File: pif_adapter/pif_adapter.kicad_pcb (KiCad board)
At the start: 2 copper layers, 11 x 22 mm, 11 parts, among them P1 Conn_02x20_Odd_Even, P10 Conn_01x01, P11 Conn_01x01, P2 PIF-NUS, P3 Conn_01x01, P4 Conn_01x01, P5 Conn_01x01, P6 Conn_01x01, P7 Conn_01x01, P8 Conn_01x01, P9 Conn_01x01

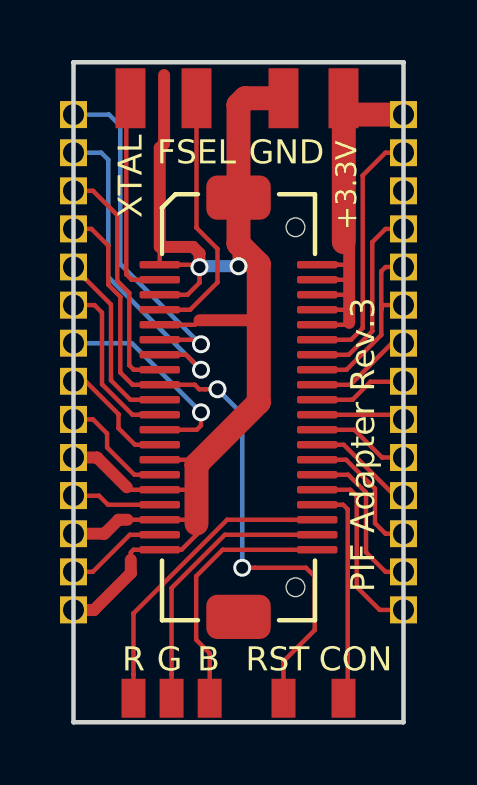
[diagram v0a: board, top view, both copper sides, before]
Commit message: - updated revision infos - changed some traces
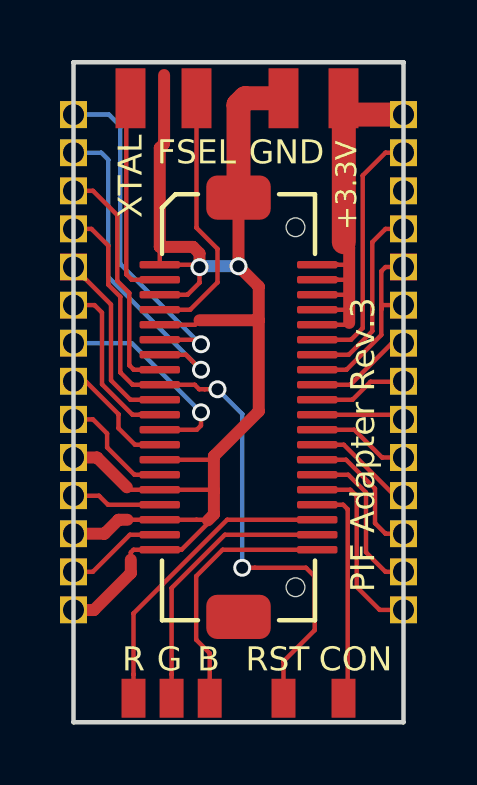
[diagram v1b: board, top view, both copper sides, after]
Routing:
- net GND: track 51.8 -> 51.1 mm
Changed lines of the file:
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@@
     (thickness 1.6)
     (drawings 20)
-    (tracks 221)
+    (tracks 222)
     (zones 0)
     (modules 11)
@@
   )
   (page A4)
+  (title_block
+    (title "UltraPIF Adapter")
+    (date 2020-03-04)
+    (rev 3)
+  )
   (layers
     (0 F.Cu signal)
@@
   )
   (setup
-    (last_trace_width 0.8)
+    (last_trace_width 0.4)
     (user_trace_width 0.4)
     (user_trace_width 0.8)
@@
   (segment (start 143.03 109.25) (end 142.12 108.34) (width 0.15) (layer F.Cu) (net 9))
   (segment (start 141.01 111.225) (end 141 111.215) (width 0.15) (layer F.Cu) (net 10))
-  (segment (start 143.975 110.75) (end 142.8 110.75) (width 0.15) (layer F.Cu) (net 10))
   (segment (start 141 111.215) (end 142.035 111.215) (width 0.4) (layer F.Cu) (net 10))
   (segment (start 142.5 110.75) (end 142.8 110.75) (width 0.4) (layer F.Cu) (net 10))
   (segment (start 142.035 111.215) (end 142.5 110.75) (width 0.4) (layer F.Cu) (net 10))
-  (segment (start 143.975 108.75) (end 144.925 108.75) (width 0.15) (layer F.Cu) (net 10))
   (via (at 146.5 102.3) (size 0.6) (drill 0.4) (layers F.Cu B.Cu) (net 10))
   (segment (start 145.2 102.3) (end 146.5 102.3) (width 0.4) (layer B.Cu) (net 10))
@@
   (segment (start 143.975 103.25) (end 144.8 103.25) (width 0.15) (layer F.Cu) (net 10))
   (segment (start 145.2 102.85) (end 145.2 102.3) (width 0.15) (layer F.Cu) (net 10))
-  (segment (start 143.975 110.75) (end 145.1 110.75) (width 0.15) (layer F.Cu) (net 10))
-  (segment (start 145.1 111.25) (end 144.6 111.75) (width 0.15) (layer F.Cu) (net 10))
-  (segment (start 145.1 111.1) (end 145.1 111.25) (width 0.15) (layer F.Cu) (net 10))
-  (segment (start 144.6 111.75) (end 143.975 111.75) (width 0.15) (layer F.Cu) (net 10))
-  (segment (start 147.2 102.3) (end 146.5 102.3) (width 0.4) (layer F.Cu) (net 10))
   (segment (start 141.785 108.675) (end 142.78 109.67) (width 0.4) (layer F.Cu) (net 10))
   (segment (start 141 108.675) (end 141.785 108.675) (width 0.4) (layer F.Cu) (net 10))
-  (segment (start 142.86 109.75) (end 142.78 109.67) (width 0.15) (layer F.Cu) (net 10))
-  (segment (start 143.925 109.75) (end 142.86 109.75) (width 0.15) (layer F.Cu) (net 10))
-  (segment (start 144.75 109.75) (end 145.1 109.75) (width 0.15) (layer F.Cu) (net 10))
-  (segment (start 143.925 109.75) (end 144.75 109.75) (width 0.15) (layer F.Cu) (net 10))
   (segment (start 141.005 113.76) (end 141 113.755) (width 0.4) (layer F.Cu) (net 10))
   (segment (start 142.91 112.53) (end 141.68 113.76) (width 0.4) (layer F.Cu) (net 10))
@@
   (segment (start 142.91 112.53) (end 142.91 112.08) (width 0.4) (layer F.Cu) (net 10))
   (segment (start 142.91 112.08) (end 142.91 111.84) (width 0.15) (layer F.Cu) (net 10))
-  (segment (start 147.2 104.1) (end 145.2 104.1) (width 0.4) (layer F.Cu) (net 10))
-  (segment (start 147.212501 104.087499) (end 147.2 104.1) (width 0.4) (layer F.Cu) (net 10))
   (segment (start 145.2 104.1) (end 145.4 104.1) (width 0.15) (layer F.Cu) (net 10))
   (segment (start 143.975 104.25) (end 145.05 104.25) (width 0.15) (layer F.Cu) (net 10))
   (segment (start 145.05 104.25) (end 145.2 104.1) (width 0.15) (layer F.Cu) (net 10))
-  (segment (start 147.2 102.3) (end 147.212501 102.312501) (width 0.4) (layer F.Cu) (net 10))
   (segment (start 146.5 102.3) (end 146.5 100.1) (width 0.4) (layer F.Cu) (net 10))
   (segment (start 146.5 96.92) (end 146.5 100.1) (width 0.8) (layer F.Cu) (net 10))
   (segment (start 148 96.7) (end 146.72 96.7) (width 0.8) (layer F.Cu) (net 10))
   (segment (start 146.72 96.7) (end 146.5 96.92) (width 0.8) (layer F.Cu) (net 10))
-  (segment (start 144.02 98.21) (end 144.02 95.92501) (width 0.4) (layer F.Cu) (net 10))
-  (segment (start 143.875 98.355) (end 144.02 98.21) (width 0.4) (layer F.Cu) (net 10))
-  (segment (start 143.875 101.655) (end 143.875 98.355) (width 0.4) (layer F.Cu) (net 10))
   (segment (start 143.875 101.655) (end 143.875 102.25) (width 0.15) (layer F.Cu) (net 10))
   (segment (start 144.985 101.655) (end 145.2 101.87) (width 0.4) (layer F.Cu) (net 10))
   (segment (start 143.875 101.655) (end 144.985 101.655) (width 0.4) (layer F.Cu) (net 10))
   (segment (start 145.2 101.87) (end 145.2 102.33) (width 0.4) (layer F.Cu) (net 10))
-  (segment (start 147.175 106.835) (end 145.1 108.91) (width 0.8) (layer F.Cu) (net 10))
-  (segment (start 147.175 102.225) (end 147.175 106.835) (width 0.8) (layer F.Cu) (net 10))
-  (segment (start 146.5 100.1) (end 146.5 101.55) (width 0.8) (layer F.Cu) (net 10))
-  (segment (start 145.1 108.91) (end 145.1 110.88) (width 0.8) (layer F.Cu) (net 10))
-  (segment (start 146.5 101.55) (end 147.175 102.225) (width 0.8) (layer F.Cu) (net 10))
+  (segment (start 145.1 110.75) (end 143.975 110.75) (width 0.15) (layer F.Cu) (net 10))
+  (segment (start 143.975 110.75) (end 142.8 110.75) (width 0.15) (layer F.Cu) (net 10))
+  (segment (start 145.5 110.75) (end 145.68 110.57) (width 0.15) (layer F.Cu) (net 10))
+  (segment (start 145.1 110.75) (end 145.5 110.75) (width 0.15) (layer F.Cu) (net 10))
+  (segment (start 145.68 108.63) (end 145.68 109.78) (width 0.4) (layer F.Cu) (net 10))
+  (segment (start 145.68 109.78) (end 145.68 110.57) (width 0.4) (layer F.Cu) (net 10))
+  (segment (start 142.86 109.75) (end 142.78 109.67) (width 0.15) (layer F.Cu) (net 10))
+  (segment (start 145.68 109.78) (end 145.65 109.75) (width 0.15) (layer F.Cu) (net 10))
+  (segment (start 145.65 109.75) (end 142.86 109.75) (width 0.15) (layer F.Cu) (net 10))
+  (segment (start 145.56 108.75) (end 145.68 108.63) (width 0.15) (layer F.Cu) (net 10))
+  (segment (start 143.975 108.75) (end 145.56 108.75) (width 0.15) (layer F.Cu) (net 10))
+  (segment (start 145.48 110.87) (end 145.48 110.77) (width 0.15) (layer F.Cu) (net 10))
+  (segment (start 143.975 111.75) (end 144.6 111.75) (width 0.15) (layer F.Cu) (net 10))
+  (segment (start 144.6 111.75) (end 145.48 110.87) (width 0.15) (layer F.Cu) (net 10))
+  (segment (start 145.68 110.57) (end 145.48 110.77) (width 0.4) (layer F.Cu) (net 10))
+  (segment (start 147.17 104.1) (end 145.2 104.1) (width 0.4) (layer F.Cu) (net 10))
+  (segment (start 147.175 104.105) (end 147.17 104.1) (width 0.4) (layer F.Cu) (net 10))
+  (segment (start 147.175 107.135) (end 145.68 108.63) (width 0.4) (layer F.Cu) (net 10))
+  (segment (start 146.5 102.3) (end 147.175 102.975) (width 0.4) (layer F.Cu) (net 10))
+  (segment (start 147.175 102.975) (end 147.175 107.135) (width 0.4) (layer F.Cu) (net 10))
+  (segment (start 143.875 98.355) (end 144.02 98.21) (width 0.4) (layer F.Cu) (net 10))
+  (segment (start 143.875 101.655) (end 143.875 98.355) (width 0.4) (layer F.Cu) (net 10))
+  (segment (start 144.02 98.21) (end 144.02 95.92501) (width 0.4) (layer F.Cu) (net 10))
   (segment (start 141.85 109.95) (end 141.005 109.95) (width 0.15) (layer F.Cu) (net 11))
   (segment (start 141.005 109.95) (end 141 109.945) (width 0.15) (layer F.Cu) (net 11))
